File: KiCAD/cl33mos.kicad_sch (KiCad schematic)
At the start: 13 parts, among them J1 Edge2x6_Connector, J2 USB_B_Micro, U1 ESP32-WROOM-32, U2 AMS1117-3.3

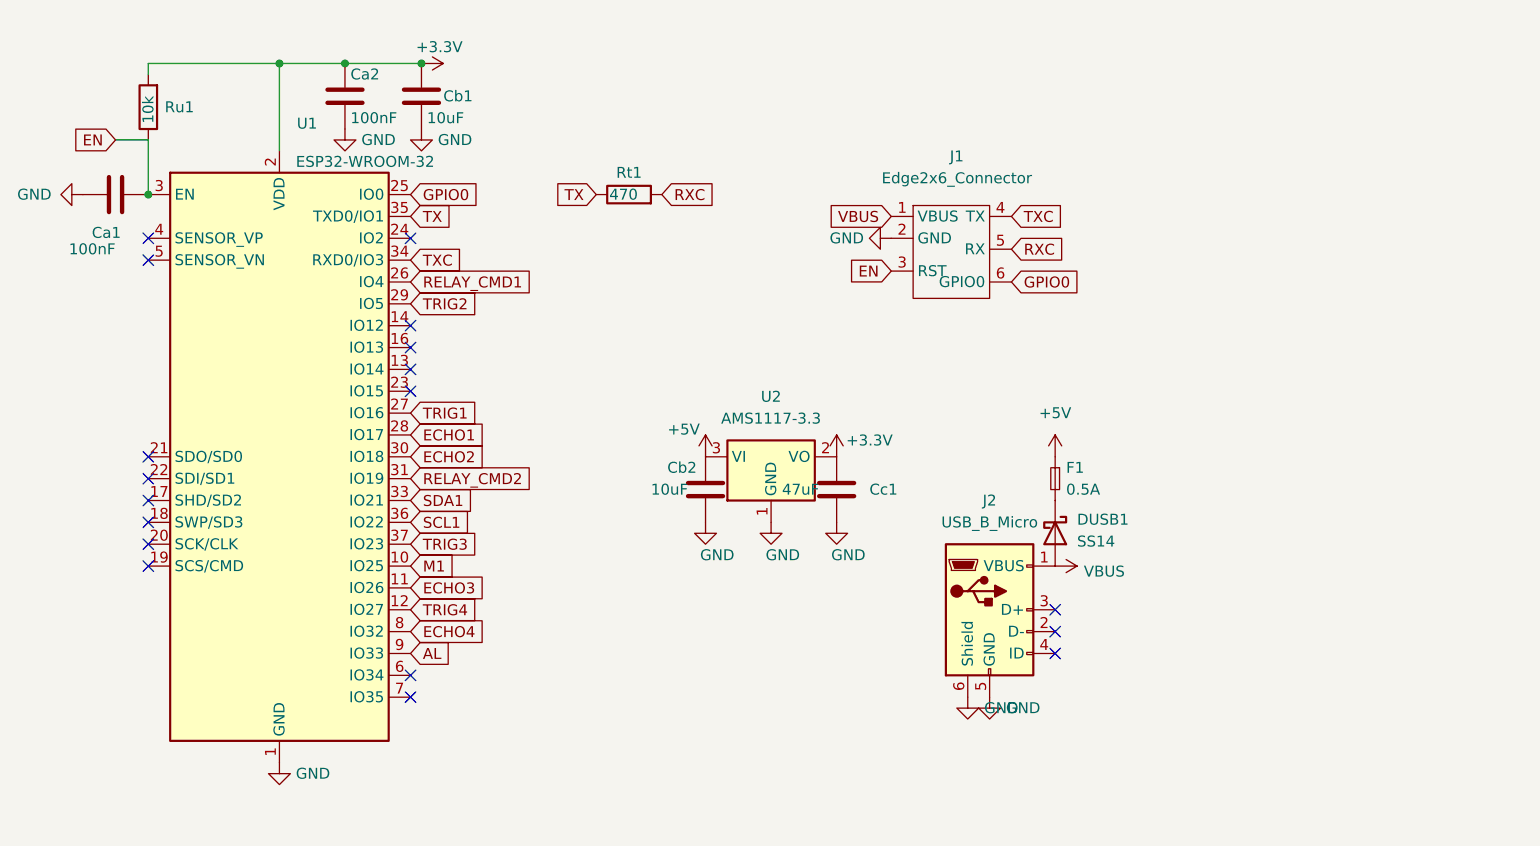
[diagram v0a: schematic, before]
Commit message: KiCAD board v3.0 changes (I think)
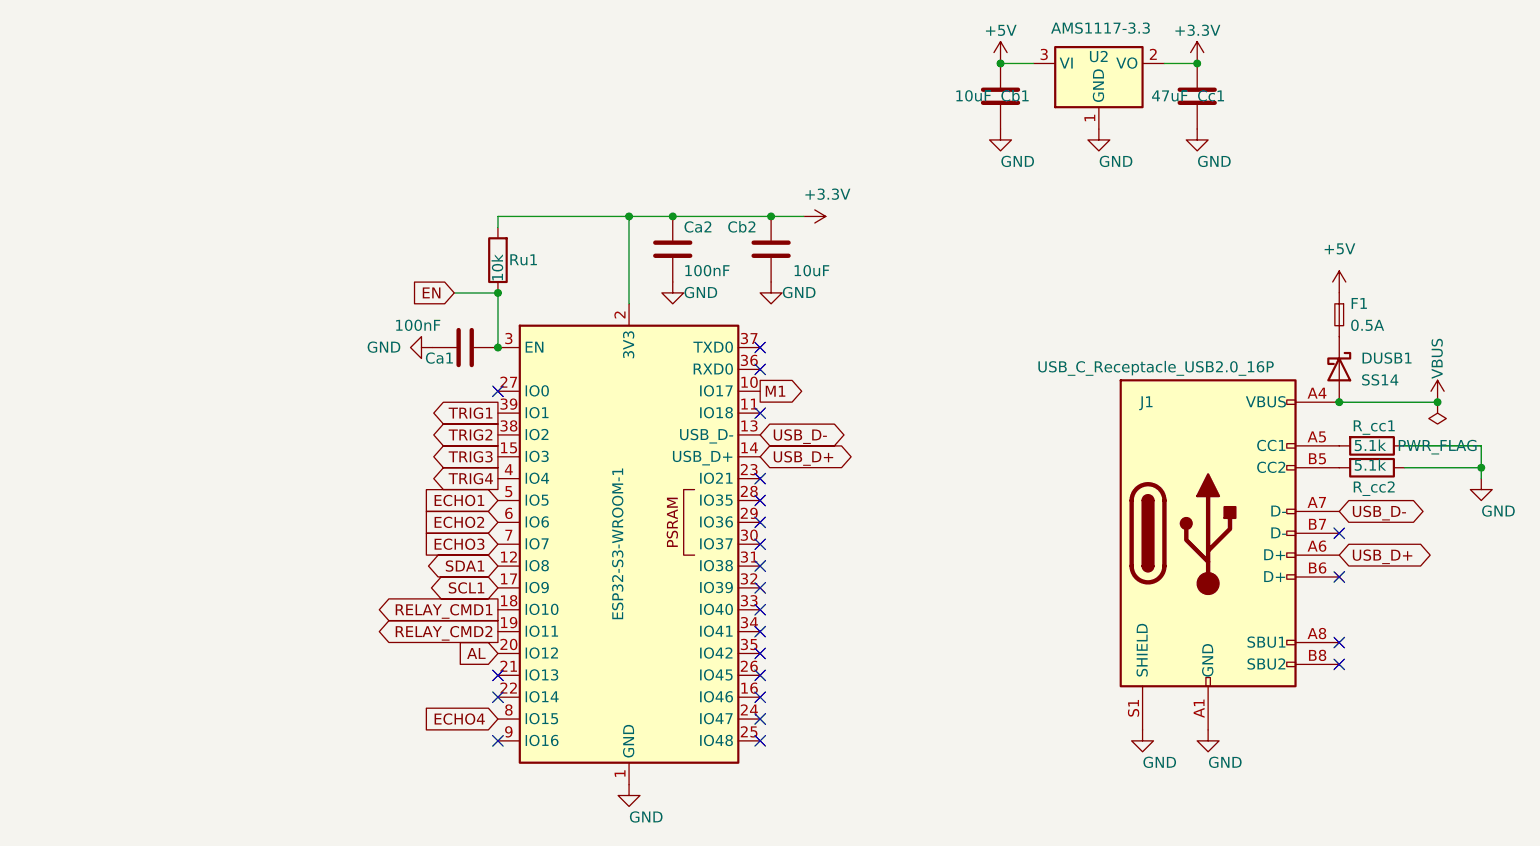
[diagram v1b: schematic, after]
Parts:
- removed J1: Edge2x6_Connector, chl33_library:EdgeConnector_2x3, symbol chl33:Edge2x6_Connector
- removed J2: USB_B_Micro, Connector_USB:USB_Micro-B_Amphenol_10118194_Horizontal, symbol Connector:USB_B_Micro
- removed Rt1: 470, Resistor_SMD:R_0603_1608Metric, symbol Device:R
- removed U1: ESP32-WROOM-32, RF_Module:ESP32-WROOM-32, symbol RF_Module:ESP32-WROOM-32
- added J1: USB_C_Receptacle_USB2.0_16P, Connector_USB:USB_C_Receptacle_HRO_TYPE-C-31-M-12, symbol Connector:USB_C_Receptacle_USB2.0_16P
- added R_cc1, R_cc2: 5.1k, Resistor_SMD:R_0603_1608Metric, symbol Device:R
- added U1: ESP32-S3-WROOM-1, RF_Module:ESP32-S3-WROOM-1, symbol RF_Module:ESP32-S3-WROOM-1
- DUSB1: footprint Diode_SMD:D_2010_5025Metric -> Diode_SMD:D_SMA
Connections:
- net +3.3V: now also Cb2.1, U1.2 (3V3); no longer Cb1.1
- net +5V: now also Cb1.1; no longer Cb2.1
- net AL: now also U1.20 (IO12)
- net ECHO1: now also U1.5 (IO5)
- net ECHO2: now also U1.6 (IO6)
- net ECHO3: now also U1.7 (IO7)
- net ECHO4: now also U1.8 (IO15)
- net EN: now also U1.3 (EN)
- net GND: now also J1.A1 (GND), J1.A12 (GND), J1.B1 (GND), J1.B12 (GND), J1.S1 (SHIELD), R_cc1.1, R_cc2.1, U1.1 (GND), U1.40 (GND), U1.41 (GND)
- net M1: now also U1.10 (IO17)
- net RELAY_CMD1: now also U1.18 (IO10)
- net RELAY_CMD2: now also U1.19 (IO11)
- net SCL1: now also U1.17 (IO9)
- net SDA1: now also U1.12 (IO8)
- net TRIG1: now also U1.39 (IO1)
- net TRIG2: now also U1.38 (IO2)
- net TRIG3: now also U1.15 (IO3)
- net TRIG4: now also U1.4 (IO4)
- net VBUS: now also J1.A4 (VBUS), J1.A9 (VBUS), J1.B4 (VBUS), J1.B9 (VBUS)
- new net: J1.A5 (CC1), R_cc1.2
- new net: J1.B5 (CC2), R_cc2.2
- new net USB_D+: J1.A6 (D+), U1.14 (USB_D+)
- new net USB_D-: J1.A7 (D-), U1.13 (USB_D-)
- no-connect marks 18 -> 24
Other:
- moved on the sheet: Ca1, Ca2, Cb1, Cb2, Cc1, DUSB1, F1, Ru1, U2
